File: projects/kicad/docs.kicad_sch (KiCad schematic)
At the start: 21 parts, among them J1 Micro_SD_Card, SW1 SW_PUSH, SW2 SW_PUSH, SW3 SW_PUSH, SW4 SW_PUSH, SW5 SW_PUSH, SW6 SW_PUSH, SW7 RotaryEncoder_Switch, U1 Pico, U2 LCD

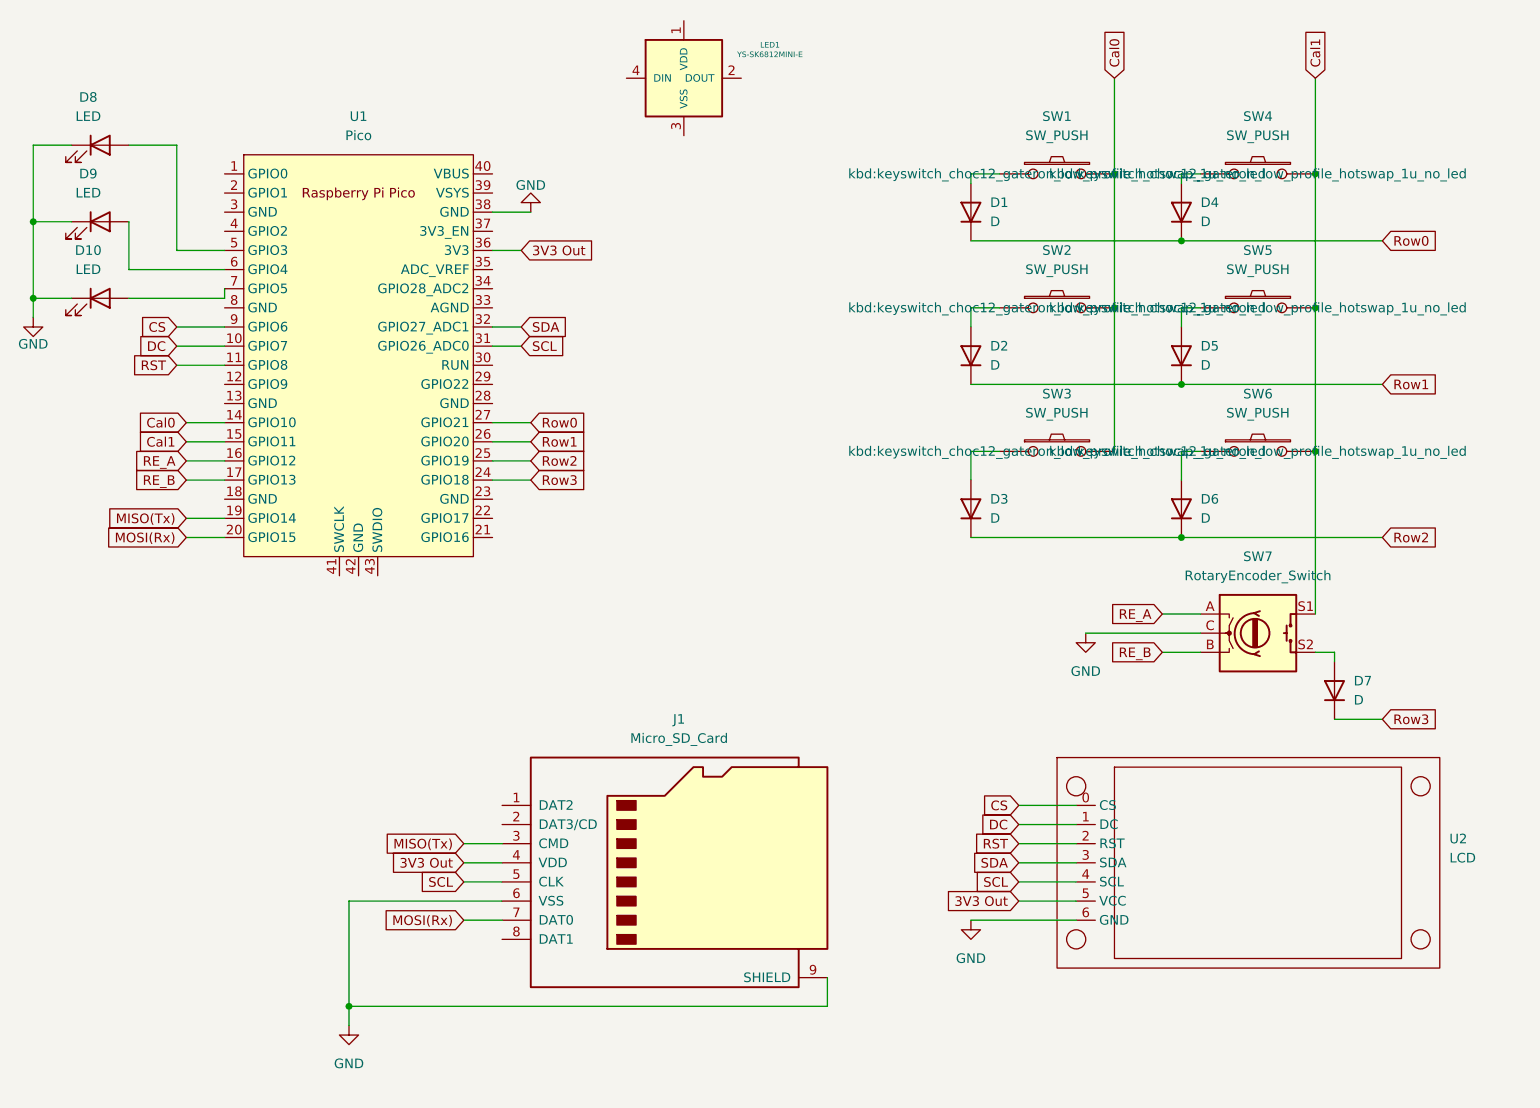
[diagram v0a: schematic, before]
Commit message: Update_0128
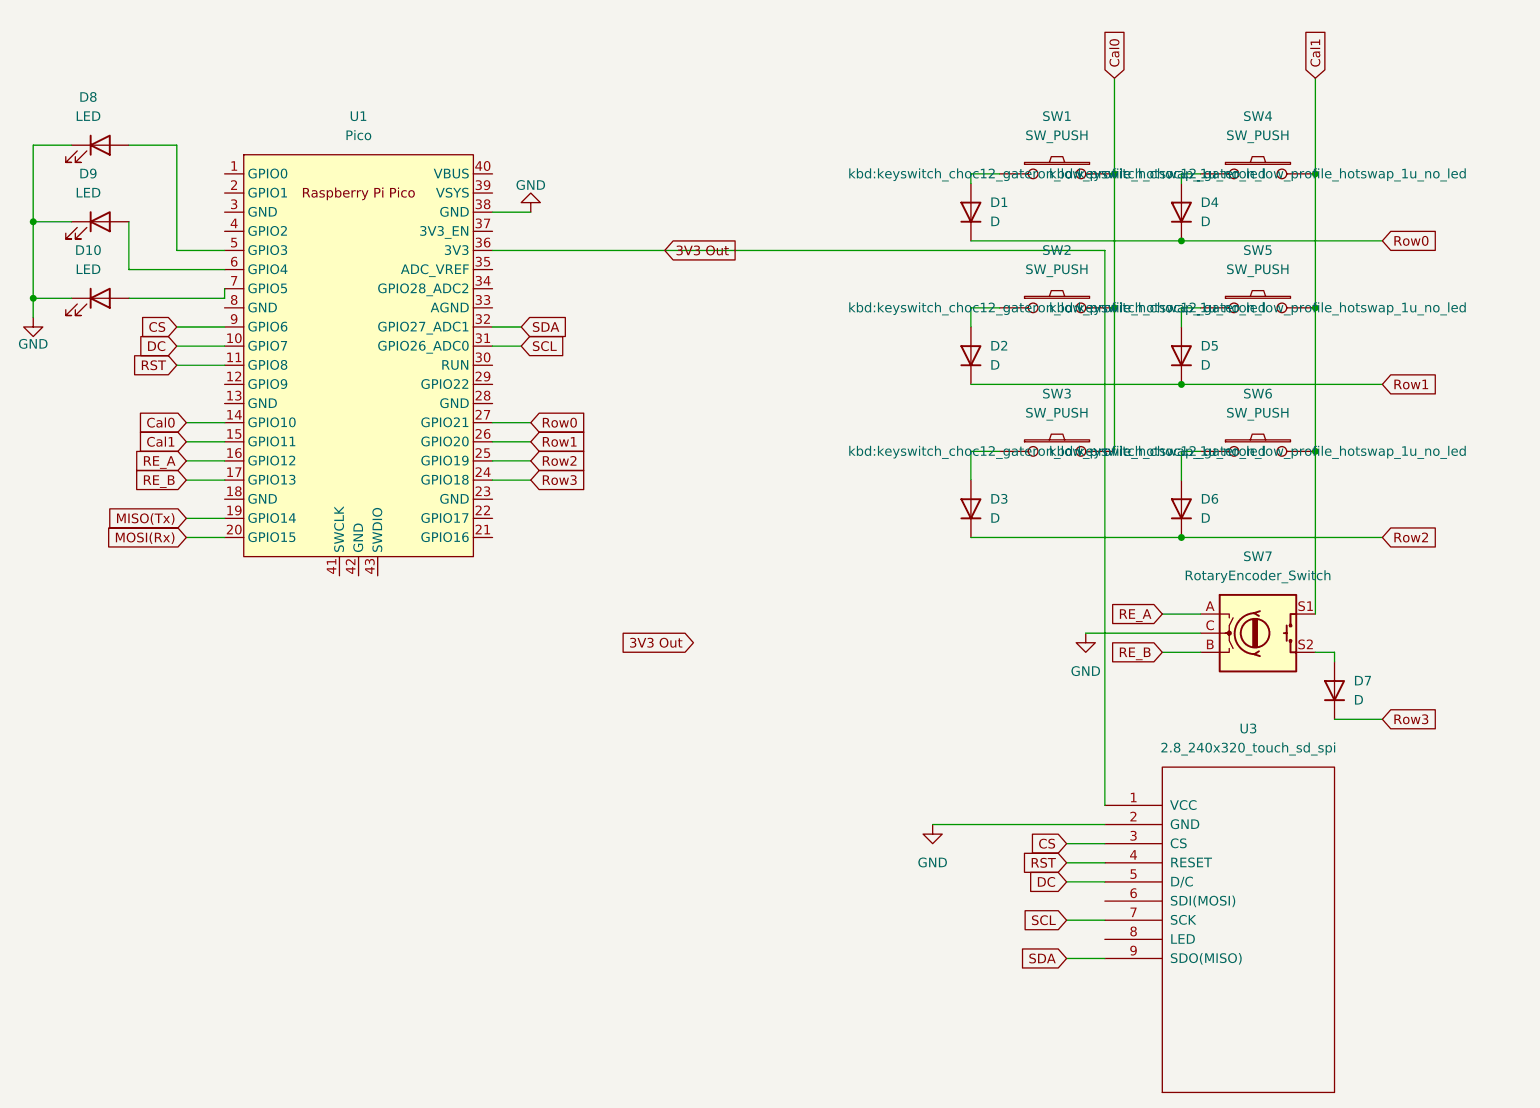
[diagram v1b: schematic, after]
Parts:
- removed J1: Micro_SD_Card, symbol Connector:Micro_SD_Card
- removed LED1: YS-SK6812MINI-E, symbol kbd:YS-SK6812MINI-E
- removed U2: LCD, tft_displays:2.8_tft_240x320_touch_sd_spi, symbol 4xxx_IEEE:4001
- added U3: 2.8_240x320_touch_sd_spi, original_tft_display:2.8_tft_240x320_touch_sd_spi, symbol TFT Displays:2.8_240x320_touch_sd_spi
- U1: footprint RPi_Pico:RPi_Pico_SMD_TH -> KiCad-RP-Pico-main:RPi_Pico_SMD_TH
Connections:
- net 3V3 Out: now also U3.1 (VCC)
- net CS: now also U3.3 (CS)
- net DC: now also U3.5 (D/C)
- net GND: now also U3.2 (GND)
- net RST: now also U3.4 (RESET)
- net SCL: now also U3.7 (SCK)
- net SDA: now also U3.9 (SDO(MISO))

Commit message: Update_0129
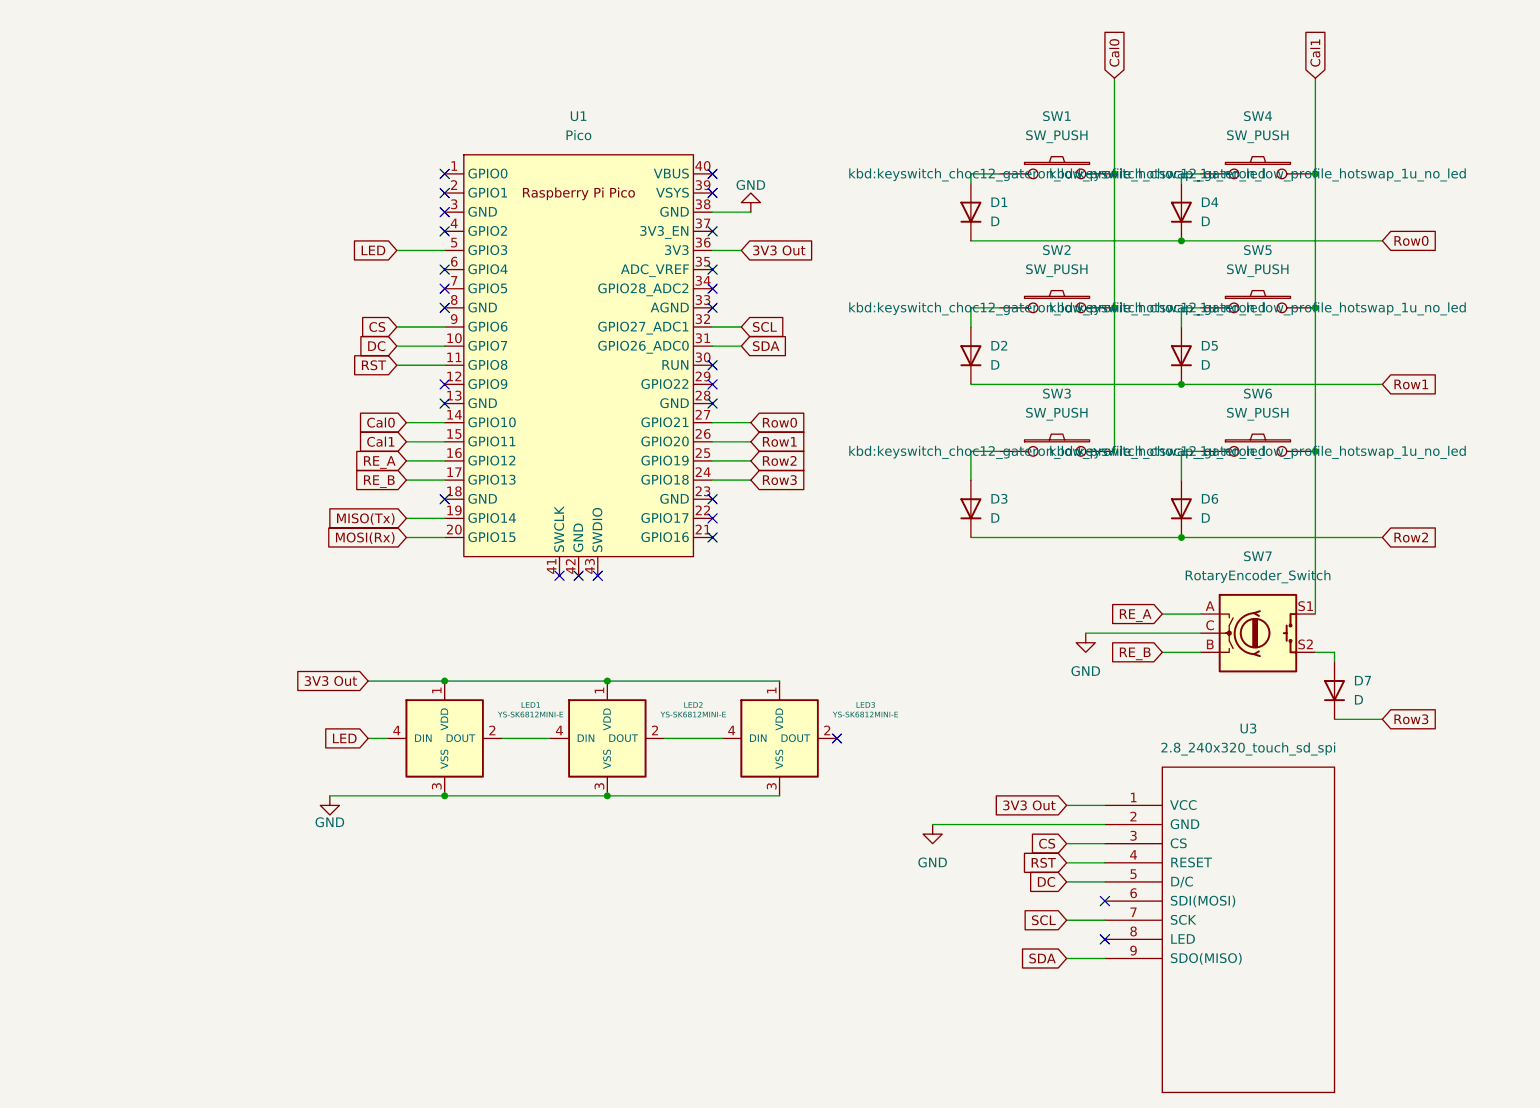
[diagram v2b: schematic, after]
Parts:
- removed D10, D8, D9: LED, kbd:LED_WS2812B-PLCC4, symbol Device:LED
- added LED1, LED2, LED3: YS-SK6812MINI-E, kbd:YS-SK6812MINI-E, symbol kbd:YS-SK6812MINI-E
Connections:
- net 3V3 Out: now also LED1.1 (VDD), LED2.1 (VDD), LED3.1 (VDD)
- net GND: now also LED1.3 (VSS), LED2.3 (VSS), LED3.3 (VSS)
- net SCL: now also U1.32 (GPIO27_ADC1); no longer U1.31 (GPIO26_ADC0)
- net SDA: now also U1.31 (GPIO26_ADC0); no longer U1.32 (GPIO27_ADC1)
- net LED: now reaches U1.5 (GPIO3)
- net LED: now also LED1.4 (DIN)
- new net: LED2.2 (DOUT), LED3.4 (DIN)
- new net: LED1.2 (DOUT), LED2.4 (DIN)
- no-connect marks 0 -> 28
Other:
- moved on the sheet: U1
